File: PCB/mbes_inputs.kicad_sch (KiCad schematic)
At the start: 28 parts, among them Q1 BC337, Q2 BC337, U3 TL084

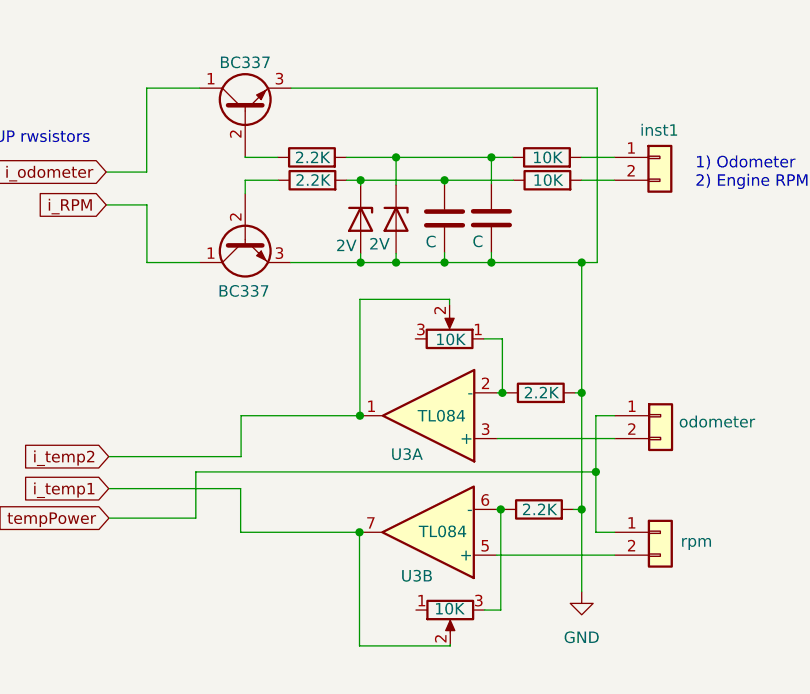
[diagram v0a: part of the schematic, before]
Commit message: fix
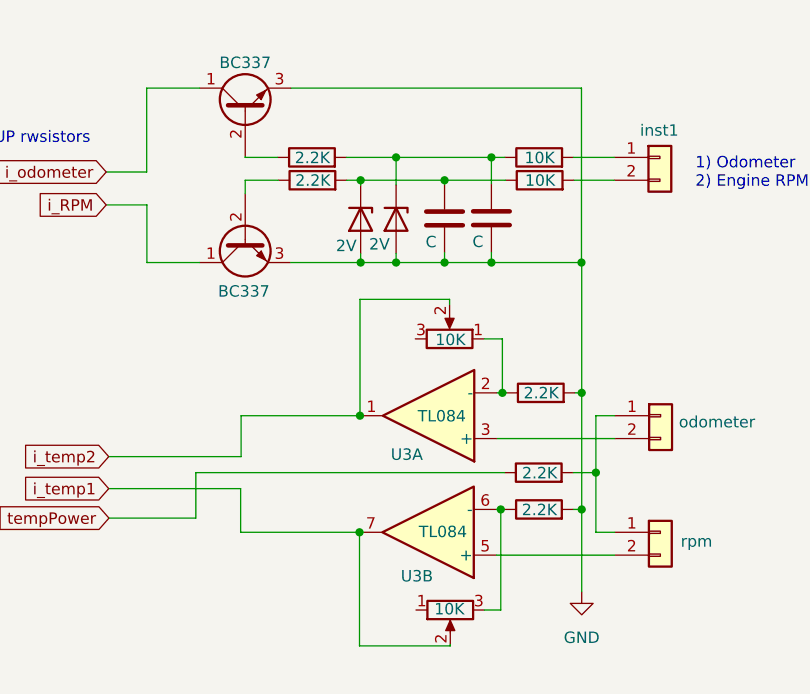
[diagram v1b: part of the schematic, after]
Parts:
- added R17: 2.2K, symbol Device:R
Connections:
- net tempPower: now also R17.1; no longer j?.1 (Pin_1), j?.1 (Pin_1)
- new net: R17.2, j?.1 (Pin_1), j?.1 (Pin_1)
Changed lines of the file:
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@@
   (junction (at 211.0994 94.6912) (diameter 0) (color 0 0 0 0)
   )
-  (junction (at 237.363 87.9856) (diameter 0) (color 0 0 0 0)
-  )
   (junction (at 220.5482 64.7192) (diameter 0) (color 0 0 0 0)
   )
@@
   (junction (at 215.1634 53.0352) (diameter 0) (color 0 0 0 0)
   )
-  (junction (at 235.7882 64.7192) (diameter 0) (color 0 0 0 0)
+  (junction (at 235.7628 64.7192) (diameter 0) (color 0 0 0 0)
   )
   (junction (at 211.1502 81.7372) (diameter 0) (color 0 0 0 0)
@@
   )
   (junction (at 78.232 135.89) (diameter 0) (color 0 0 0 0)
+  )
+  (junction (at 237.363 88.0618) (diameter 0) (color 0 0 0 0)
   )
   (junction (at 211.2264 64.7192) (diameter 0) (color 0 0 0 0)
@@
     (stroke (width 0) (type default))
   )
-  (wire (pts (xy 237.363 94.6912) (xy 237.363 87.9856))
+  (wire (pts (xy 237.363 94.6912) (xy 237.363 88.0618))
     (stroke (width 0) (type default))
   )
@@
     (stroke (width 0) (type default))
   )
-  (wire (pts (xy 235.7374 53.0352) (xy 239.395 53.0352))
+  (wire (pts (xy 234.8738 53.0352) (xy 239.395 53.0352))
     (stroke (width 0) (type default))
   )
@@
     (stroke (width 0) (type default))
   )
-  (wire (pts (xy 192.913 93.1164) (xy 192.913 87.9856))
+  (wire (pts (xy 192.913 93.1164) (xy 192.913 88.0618))
     (stroke (width 0) (type default))
   )
@@
     (stroke (width 0) (type default))
   )
-  (wire (pts (xy 220.5482 55.5752) (xy 228.1682 55.5752))
+  (wire (pts (xy 220.5482 55.5752) (xy 227.3046 55.5752))
     (stroke (width 0) (type default))
   )
@@
     (stroke (width 0) (type default))
   )
-  (wire (pts (xy 237.5154 45.339) (xy 237.5154 64.7192))
+  (wire (pts (xy 235.7628 45.339) (xy 235.7628 64.7192))
     (stroke (width 0) (type default))
   )
@@
     (stroke (width 0) (type default))
   )
-  (wire (pts (xy 225.7552 53.0352) (xy 228.1174 53.0352))
+  (wire (pts (xy 225.7552 53.0352) (xy 227.2538 53.0352))
     (stroke (width 0) (type default))
   )
@@
     (stroke (width 0) (type default))
   )
-  (wire (pts (xy 235.7882 64.7192) (xy 237.5154 64.7192))
-    (stroke (width 0) (type default))
-  )
   (wire (pts (xy 61.976 114.3) (xy 77.978 114.3))
     (stroke (width 0) (type default))
@@
     (stroke (width 0) (type default))
   )
-  (wire (pts (xy 235.7882 55.5752) (xy 239.395 55.5752))
+  (wire (pts (xy 234.9246 55.5752) (xy 239.395 55.5752))
     (stroke (width 0) (type default))
   )
@@
     (stroke (width 0) (type default))
   )
-  (wire (pts (xy 192.913 87.9856) (xy 237.363 87.9856))
+  (wire (pts (xy 192.913 88.0618) (xy 227.203 88.0618))
     (stroke (width 0) (type default))
   )
@@
     (stroke (width 0) (type default))
   )
-  (wire (pts (xy 237.363 87.9856) (xy 237.363 81.7372))
+  (wire (pts (xy 237.363 81.7372) (xy 237.363 88.0618))
     (stroke (width 0) (type default))
   )
@@
     (stroke (width 0) (type default))
   )
-  (wire (pts (xy 203.5048 45.339) (xy 237.5154 45.339))
+  (wire (pts (xy 203.5048 45.339) (xy 235.7628 45.339))
     (stroke (width 0) (type default))
   )
@@
     (stroke (width 0) (type default))
   )
-  (wire (pts (xy 225.7552 64.7192) (xy 235.7882 64.7192))
+  (wire (pts (xy 225.7552 64.7192) (xy 235.7628 64.7192))
+    (stroke (width 0) (type default))
+  )
+  (wire (pts (xy 234.823 88.0618) (xy 237.363 88.0618))
     (stroke (width 0) (type default))
   )
@@
   )
   (wire (pts (xy 235.7882 79.1972) (xy 235.7882 64.7192))
+    (stroke (width 0) (type default))
+  )
+  (wire (pts (xy 235.7628 64.7192) (xy 235.7882 64.7192))
     (stroke (width 0) (type default))
   )
@@
     )
   )
+  (symbol (lib_id "Device:R") (at 231.013 88.0618 90) (unit 1)
+    (in_bom yes) (on_board yes) (dnp no)
+    (property "Reference" "R17" (at 231.013 82.1182 90)
+      (effects (font (size 1.27 1.27)) hide)
+    )
+    (property "Value" "2.2K" (at 231.1146 88.1126 90)
+      (effects (font (size 1.27 1.27)))
+    )
+    (property "Footprint" "" (at 231.013 89.8398 90)
+      (effects (font (size 1.27 1.27)) hide)
+    )
+    (property "Datasheet" "~" (at 231.013 88.0618 0)
+      (effects (font (size 1.27 1.27)) hide)
+    )
+    (pin "2")
+    (pin "1")
+    (instances
+      (project "pcb-a"
+        (path "/709d0967-afe5-49d3-92a5-d2bb94550bdb/0b22d592-b723-42a2-89dd-bec665c2bd26"
+          (reference "R17") (unit 1)
+        )
+      )
+    )
+  )
   (symbol (lib_id "Device:C") (at 220.5482 59.817 0) (unit 1)
     (in_bom yes) (on_board yes) (dnp no)
@@
     )
   )
-  (symbol (lib_id "Device:R") (at 231.9274 53.0352 90) (unit 1)
-    (in_bom yes) (on_board yes) (dnp no)
-    (property "Reference" "R11" (at 231.9274 47.0916 90)
-      (effects (font (size 1.27 1.27)) hide)
-    )
-    (property "Value" "10K" (at 231.9782 53.086 90)
-      (effects (font (size 1.27 1.27)))
-    )
-    (property "Footprint" "" (at 231.9274 54.8132 90)
-      (effects (font (size 1.27 1.27)) hide)
-    )
-    (property "Datasheet" "~" (at 231.9274 53.0352 0)
+  (symbol (lib_id "Device:R") (at 231.0638 53.0352 90) (unit 1)
+    (in_bom yes) (on_board yes) (dnp no)
+    (property "Reference" "R11" (at 231.0638 47.0916 90)
+      (effects (font (size 1.27 1.27)) hide)
+    )
+    (property "Value" "10K" (at 231.1146 53.086 90)
+      (effects (font (size 1.27 1.27)))
+    )
+    (property "Footprint" "" (at 231.0638 54.8132 90)
+      (effects (font (size 1.27 1.27)) hide)
+    )
+    (property "Datasheet" "~" (at 231.0638 53.0352 0)
       (effects (font (size 1.27 1.27)) hide)
     )
@@
     )
   )
-  (symbol (lib_id "Device:R") (at 231.9782 55.5752 90) (unit 1)
-    (in_bom yes) (on_board yes) (dnp no)
-    (property "Reference" "R12" (at 231.9782 49.6316 90)
-      (effects (font (size 1.27 1.27)) hide)
-    )
-    (property "Value" "10K" (at 232.029 55.6006 90)
-      (effects (font (size 1.27 1.27)))
-    )
-    (property "Footprint" "" (at 231.9782 57.3532 90)
-      (effects (font (size 1.27 1.27)) hide)
-    )
-    (property "Datasheet" "~" (at 231.9782 55.5752 0)
-      (effects (font (size 1.27 1.27)) hide)
-    )
+  (symbol (lib_id "Device:R") (at 231.1146 55.5752 90) (unit 1)
+    (in_bom yes) (on_board yes) (dnp no)
+    (property "Reference" "R12" (at 231.1146 49.6316 90)
+      (effects (font (size 1.27 1.27)) hide)
+    )
+    (property "Value" "10K" (at 231.1654 55.6006 90)
+      (effects (font (size 1.27 1.27)))
+    )
+    (property "Footprint" "" (at 231.1146 57.3532 90)
+      (effects (font (size 1.27 1.27)) hide)
+    )
+    (property "Datasheet" "~" (at 231.1146 55.5752 0)
+      (effects (font (size 1.27 1.27)) hide)
+    )
